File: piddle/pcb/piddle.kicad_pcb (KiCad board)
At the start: 2 copper layers, 133.5 x 118 mm, 68 parts, among them J1 Conn_01x03_Socket, J10 Conn_01x03_Socket, J11 Conn_01x02_Socket, J12 Conn_01x02_Socket, J13 Conn_01x02_Pin, J2 Conn_01x03_Socket, J3 Conn_01x03_Socket, J4 Conn_01x03_Socket, J5 Conn_01x03_Socket, J7 Conn_01x03_Socket, J8 Conn_01x03_Socket, J9 Conn_01x03_Socket, U1 ESP32-DevKitC, U2 INMP441

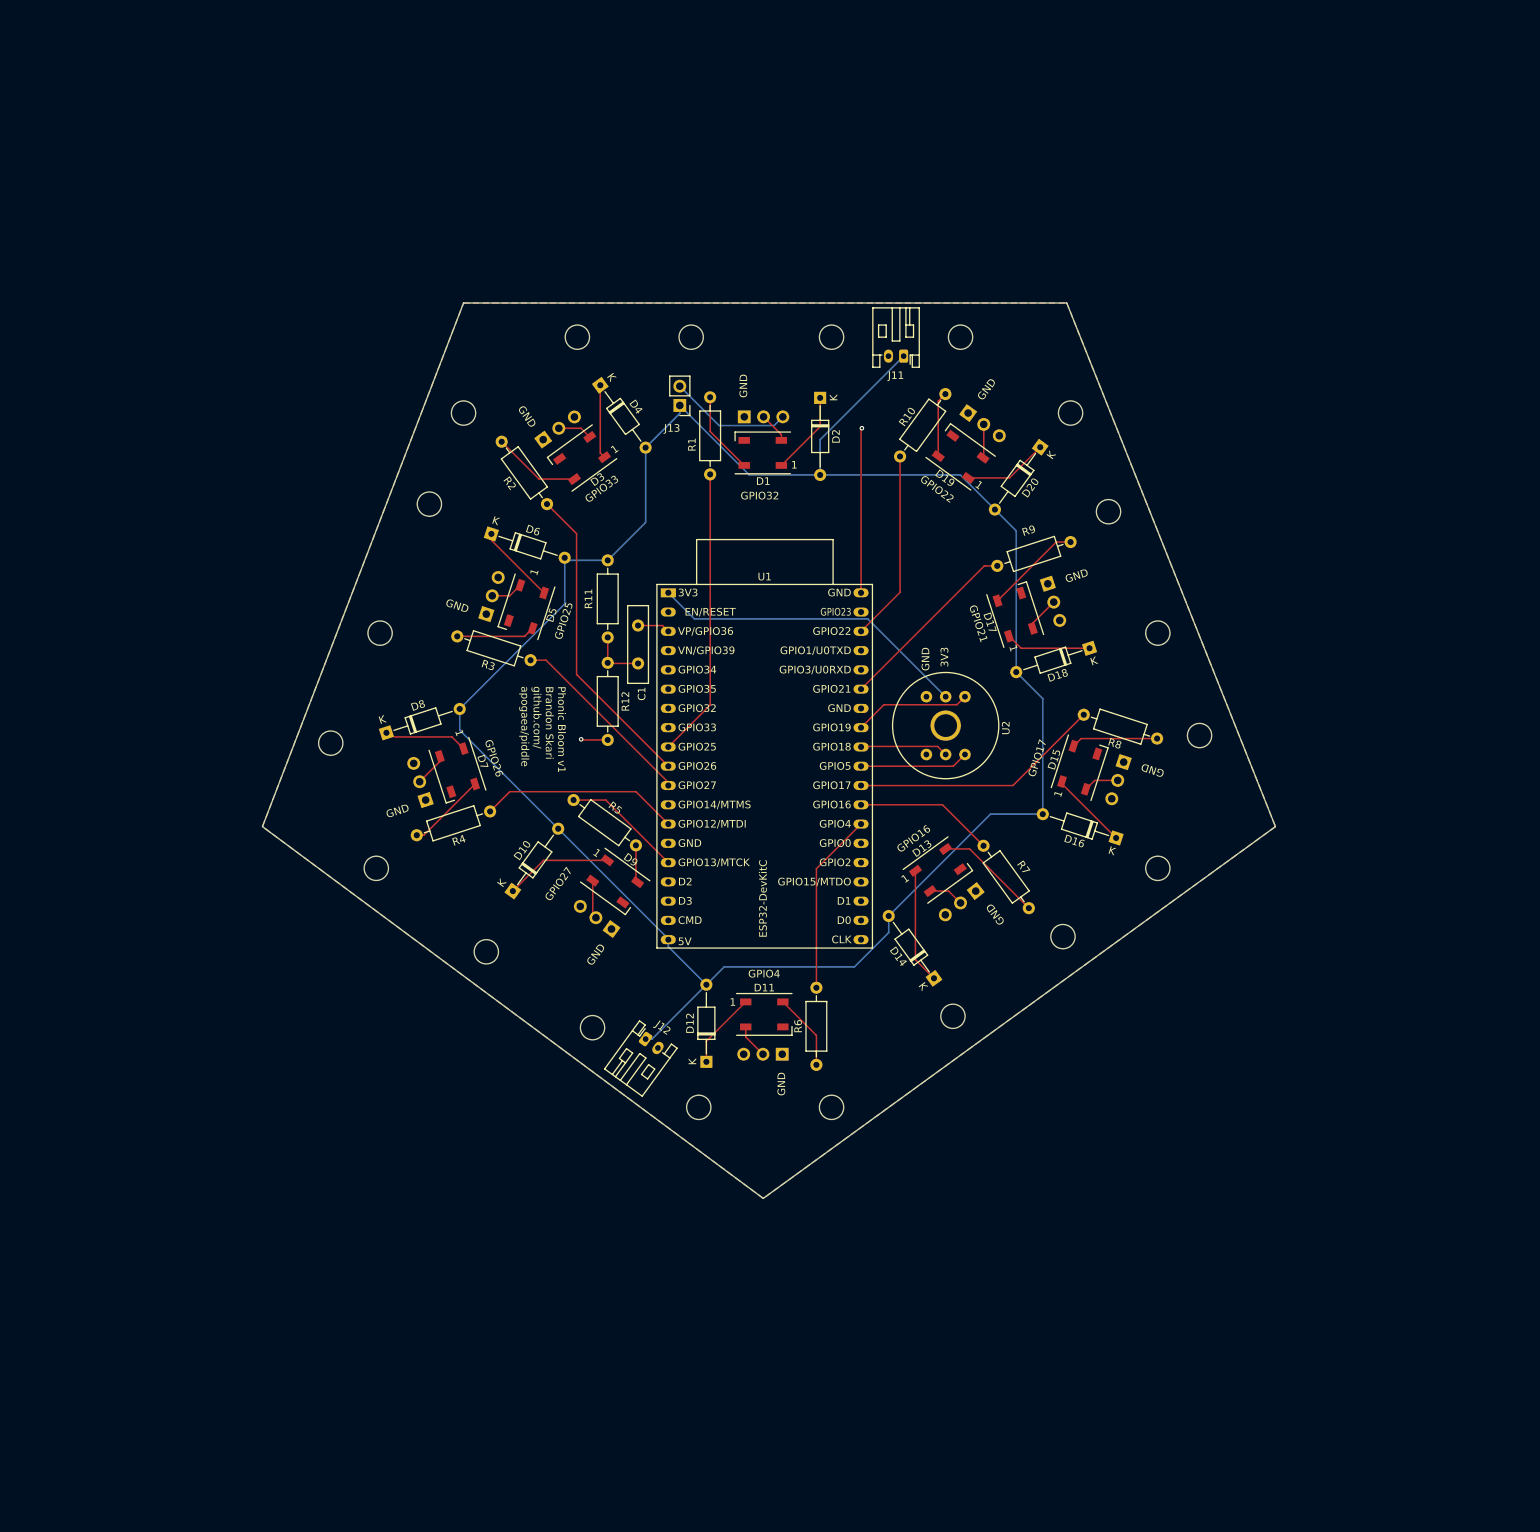
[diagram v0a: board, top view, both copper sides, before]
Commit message: Start 15 pin
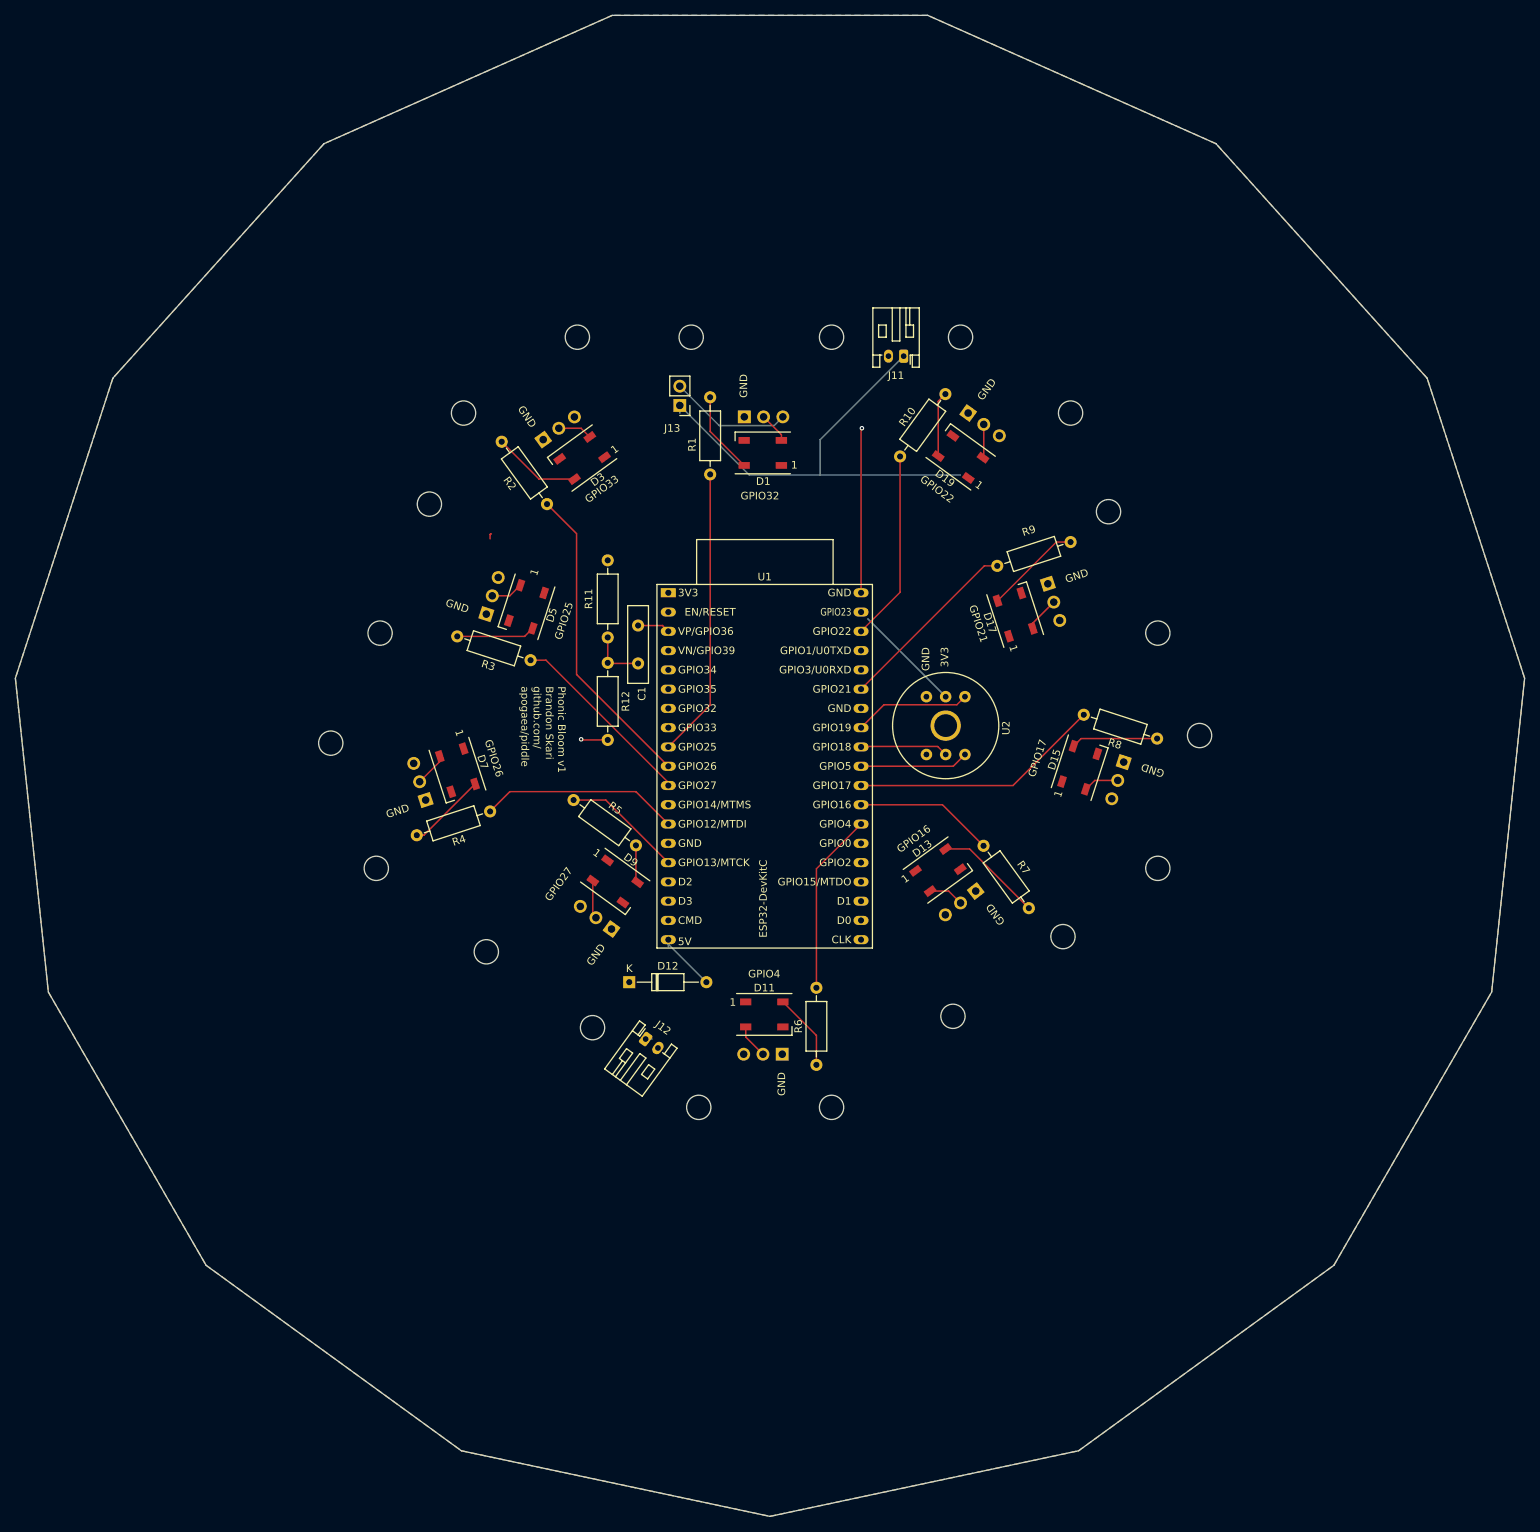
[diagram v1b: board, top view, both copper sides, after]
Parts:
- removed D10, D14, D16, D18, D2, D20, D4, D6, D8: 1N4148, Diode_THT:D_DO-35_SOD27_P10.16mm_Horizontal
- moved D12 14.6 mm to (87.5, 143.6), turned to 0 degrees
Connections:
- D1 pad 1: Net-(D1-VDD) -> /4.3V
- D11 pad 1: Net-(D11-VDD) -> /4.3V
- D12 pad 1: Net-(D11-VDD) -> /4.3V
- D13 pad 1: Net-(D13-VDD) -> /4.3V
- D15 pad 1: Net-(D15-VDD) -> /4.3V
- D17 pad 1: Net-(D17-VDD) -> /4.3V
- D19 pad 1: Net-(D19-VDD) -> /4.3V
- D3 pad 1: Net-(D3-VDD) -> /4.3V
- D5 pad 1: Net-(D5-VDD) -> /4.3V
- D7 pad 1: Net-(D7-VDD) -> /4.3V
- D9 pad 1: Net-(D10-K) -> /4.3V
- J7 pad 2: Net-(D13-DOUT) -> Net-(D13-DIN)
- R7 pad 1: Net-(D13-DIN) -> Net-(D13-DOUT)
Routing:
- net +5V: track 282.5 -> 72.3 mm
- net +3.3V: track 42.2 -> 14.5 mm
- net Net-(D13-VDD): track 15.2 -> 0.00 mm
- net Net-(D10-K): track 14.2 -> 0.00 mm
- net Net-(D5-VDD): track 11.5 -> 0.00 mm
- net Net-(D17-VDD): track 11.3 -> 0.00 mm
- net Net-(D19-VDD): track 11.2 -> 0.00 mm
- net Net-(D1-VDD): track 11.0 -> 0.00 mm
- net Net-(D15-VDD): track 10.4 -> 0.00 mm
- net Net-(D11-VDD): track 10.0 -> 0.00 mm
- net Net-(D7-VDD): track 9.78 -> 0.00 mm
- net Net-(D3-VDD): track 9.72 -> 0.00 mm
- net /4.3V: track 0.00 -> 1.70 mm
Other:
- board size 133.5 x 118 mm -> 198.9 x 197.8 mm
